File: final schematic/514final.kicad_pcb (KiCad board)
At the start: 2 copper layers, 52 x 39.5 mm, 13 parts, among them J1 3.7V Lipo Battery, U7 MLX90614ESF-BAA-000-TU

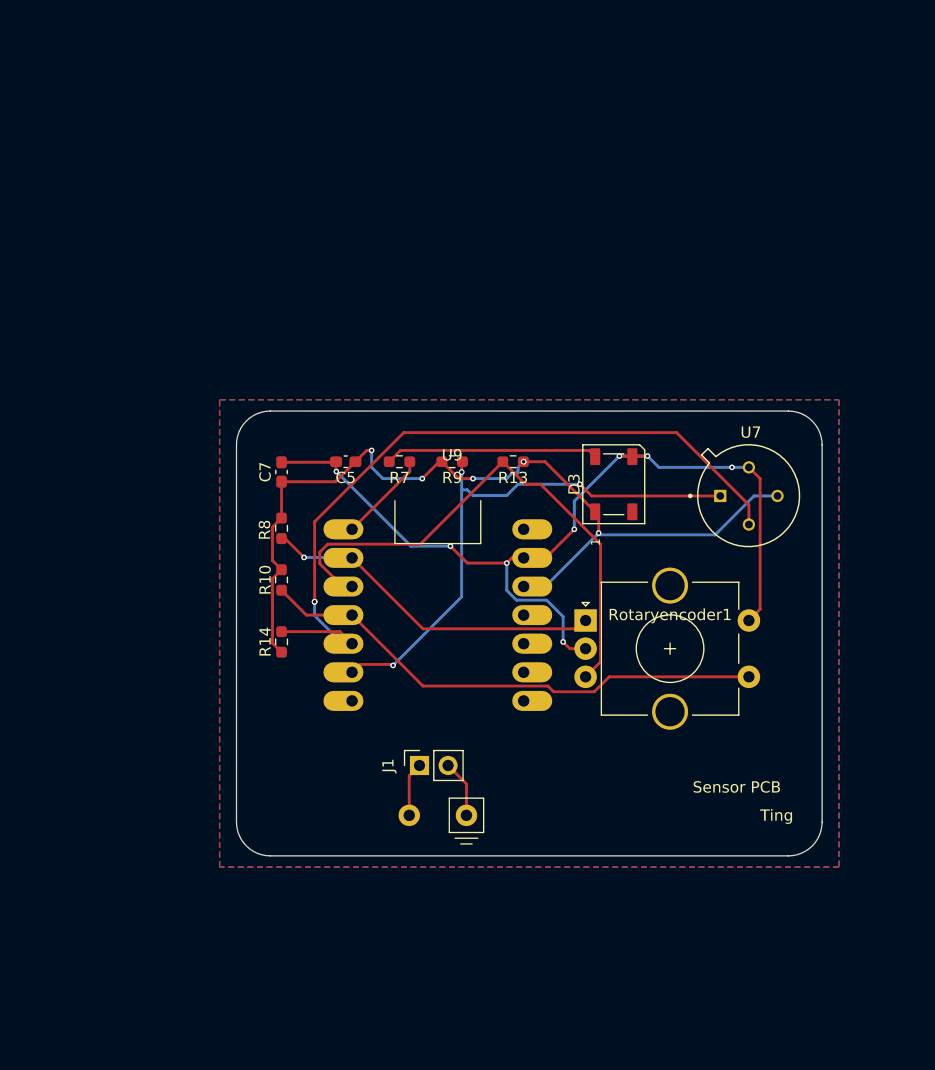
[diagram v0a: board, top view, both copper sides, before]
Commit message: add second device code
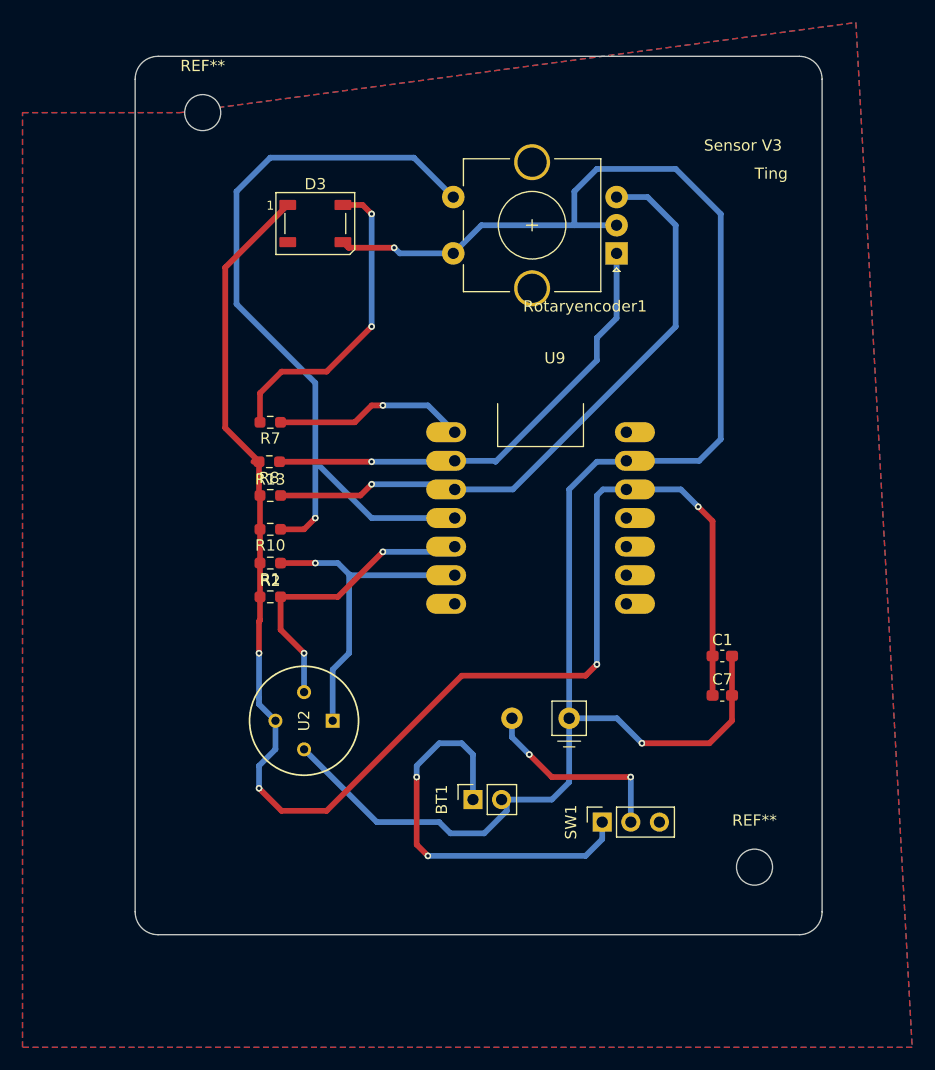
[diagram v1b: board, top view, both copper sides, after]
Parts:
- removed C5: 100nF, Capacitor_SMD:C_0603_1608Metric_Pad1.08x0.95mm_HandSolder
- removed J1: 3.7V Lipo Battery, Connector_PinSocket_2.54mm:PinSocket_1x02_P2.54mm_Vertical
- removed R14, R9: 3.3kΩ, Resistor_SMD:R_0603_1608Metric_Pad0.98x0.95mm_HandSolder
- removed U7: MLX90614ESF-BAA-000-TU, KicadFootprints:MLX90614ESF-BAA-000-4
- added BT1: Battery_Cell, Connector_PinSocket_2.54mm:PinSocket_1x02_P2.54mm_Vertical, F.Cu at (120.0, 83.0)
- added C1: 100nF, Capacitor_SMD:C_0603_1608Metric_Pad1.08x0.95mm_HandSolder, F.Cu at (142.1, 70.2)
- added R1: 3.3kΩ, Resistor_SMD:R_0603_1608Metric_Pad0.98x0.95mm_HandSolder, F.Cu at (102.0, 62.0)
- added R2: 3.3kΩ, Resistor_SMD:R_0603_1608Metric_Pad0.98x0.95mm_HandSolder, F.Cu at (102.0, 65.0)
- added REF**: MountingHole_3.2mm_M3, MountingHole:MountingHole_3.2mm_M3, F.Cu at (145.0, 89.0)
- added REF**: MountingHole_3.2mm_M3, MountingHole:MountingHole_3.2mm_M3, F.Cu at (96.0, 22.0)
- added SW1: SW_SPDT, Connector_PinSocket_2.54mm:PinSocket_1x03_P2.54mm_Vertical, F.Cu at (131.5, 85.0)
- added U2: MLX90614ESF-BAA-000-TU, 514Final:MLX90614ESF-BAA_MEL, F.Cu at (107.5, 76.0)
- U9: footprint KicadFootprints:XIAO_ESP32 -> 514Final:XIAO_ESP32
- moved C7 43.9 mm to (142.1, 73.8), turned to 0 degrees
- moved D3 35.2 mm to (106.0, 31.9), turned to 0 degrees
- moved Rotaryencoder1 32.7 mm to (132.8, 34.5), turned to 180 degrees
- moved R13 21.8 mm to (102.0, 56.0), turned to 0 degrees
- moved U9 12.5 mm to (126.0, 58.0)
- moved R7 12.0 mm to (102.0, 49.5)
- moved R8 6.01 mm to (101.9, 53.0), turned to 180 degrees
- moved R10 4.61 mm to (102.0, 59.0), turned to 180 degrees
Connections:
- U9 pad 16: Net-(J1-Pin_2) -> GND
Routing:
- net GND: track 81.4 -> 157.2 mm, vias 8 -> 2
- net +3V3: track 79.5 -> 135.5 mm, vias 5 -> 4
- net /SDA: track 65.7 -> 26.6 mm
- net Net-(BT1-+): track 0.00 -> 36.3 mm, vias 0 -> 2
- net /A3_D3: track 45.8 -> 71.8 mm, vias 0 -> 1
- net /SCL: track 48.9 -> 29.5 mm, vias 3 -> 1
- net Net-(SW1-B): track 4.80 -> 17.7 mm, vias 0 -> 2
- net /A1_D1: track 30.9 -> 42.2 mm
- net /A0_D0: track 8.12 -> 17.1 mm, vias 0 -> 1
- net Net-(D3-DIN): track 18.9 -> 27.8 mm, vias 0 -> 2
- net /A2_D2: track 48.3 -> 57.0 mm, vias 0 -> 1
- net Net-(J1-Pin_2): track 5.10 -> 0.00 mm
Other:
- board size 52 x 39.5 mm -> 61 x 78 mm
- board text added: "Sensor V3"
- board text removed: "Sensor PCB"
